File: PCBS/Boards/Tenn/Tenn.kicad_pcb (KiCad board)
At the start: 2 copper layers, 34 parts, among them J1 Conn_01x02_Socket, J10 Conn_01x03_Male, J11 Conn_01x03_Male, J12 Conn_01x04_Female, J13 Conn_01x03_Male, J14 Conn_01x03_Male, J15 Conn_01x03_Male, J16 Conn_01x02_Male, J17 Conn_01x02_Male, J2 Conn_01x03_Male, J3 Conn_01x03_Male, J4 Conn_01x03_Male, J5 Conn_01x03_Male, J6 Conn_01x03_Male, J7 Conn_01x03_Male, J8 Conn_01x03_Male, J9 Conn_01x03_Male, SW2 SW_Push, SW3 SW_Push, SW4 SW_SPDT, U1 L7805, U2 DRV8871DDA, U3 DRV8871DDA

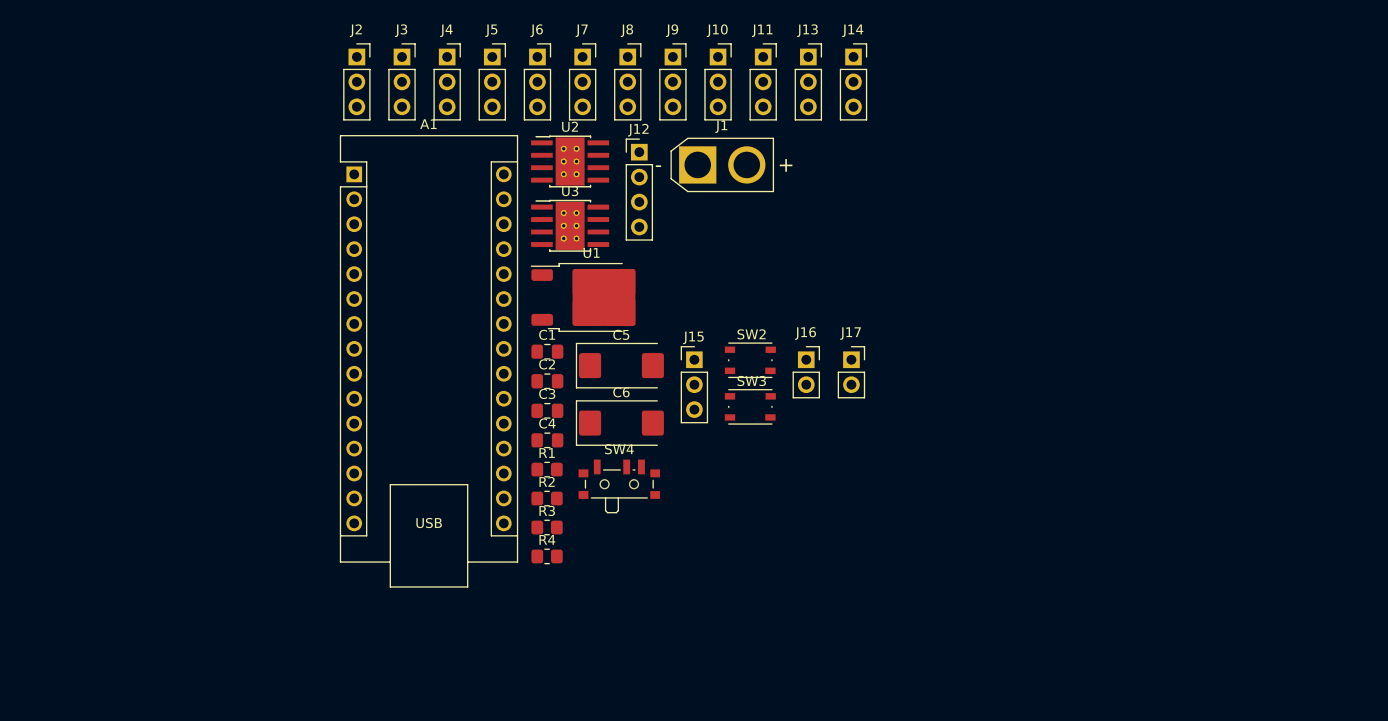
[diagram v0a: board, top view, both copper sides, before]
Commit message: updated README
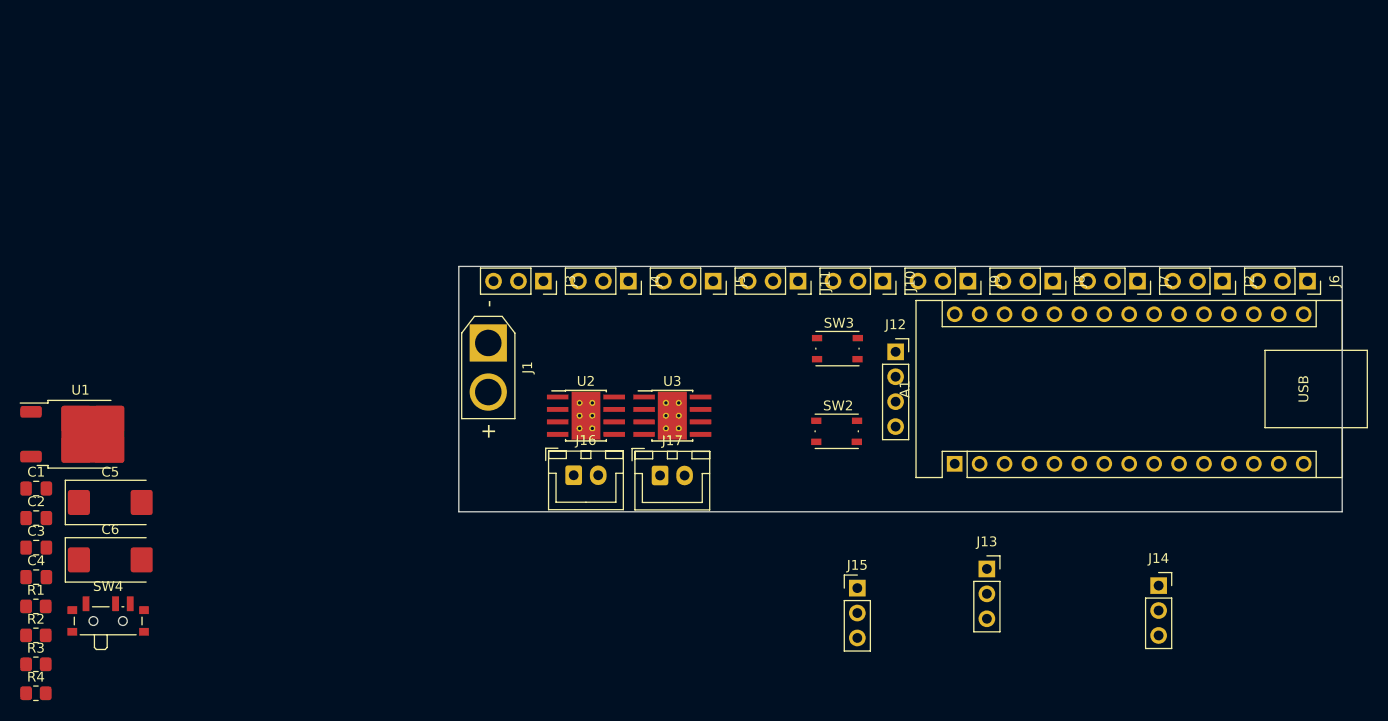
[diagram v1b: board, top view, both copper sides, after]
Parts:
- J12: footprint Connector_PinHeader_2.54mm:PinHeader_1x04_P2.54mm_Vertical -> Connector_PinSocket_2.54mm:PinSocket_1x04_P2.54mm_Vertical
- J16, J17: footprint Connector_PinSocket_2.54mm:PinSocket_1x02_P2.54mm_Vertical -> Connector_JST:JST_XH_B2B-XH-A_1x02_P2.50mm_Vertical
- moved J2 91.1 mm to (192.8, 91.2), turned to -90 degrees
- moved J6 81.7 mm to (201.5, 91.2), turned to -90 degrees
- moved A1 67.9 mm to (165.5, 109.8), turned to 90 degrees
- moved J14 62.2 mm to (186.3, 122.2)
- moved J7 61.0 mm to (184.1, 91.2), turned to -90 degrees
- moved J13 55.2 mm to (168.8, 120.5)
- moved C1 53.9 mm to (71.9, 112.3)
- moved C2 53.9 mm to (71.9, 115.3)
- moved C3 53.9 mm to (71.9, 118.3)
- moved C4 53.9 mm to (71.9, 121.4)
- moved C5 53.9 mm to (79.5, 113.8)
- moved C6 53.9 mm to (79.5, 119.6)
- moved R1 53.9 mm to (71.9, 124.3)
- moved R2 53.9 mm to (71.9, 127.3)
- moved R3 53.9 mm to (71.9, 130.2)
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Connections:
- A1 pad 21: SDA -> Sens6
- A1 pad 22: SCL -> Sens7
- A1 pad 23: Sens6 -> SDA
- A1 pad 24: Sens7 -> SCL
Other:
- board outline added: 90 x 25 mm
